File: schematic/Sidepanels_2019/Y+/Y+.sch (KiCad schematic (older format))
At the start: 42 parts, among them J1 Conn_01x04, J2 Conn_01x02

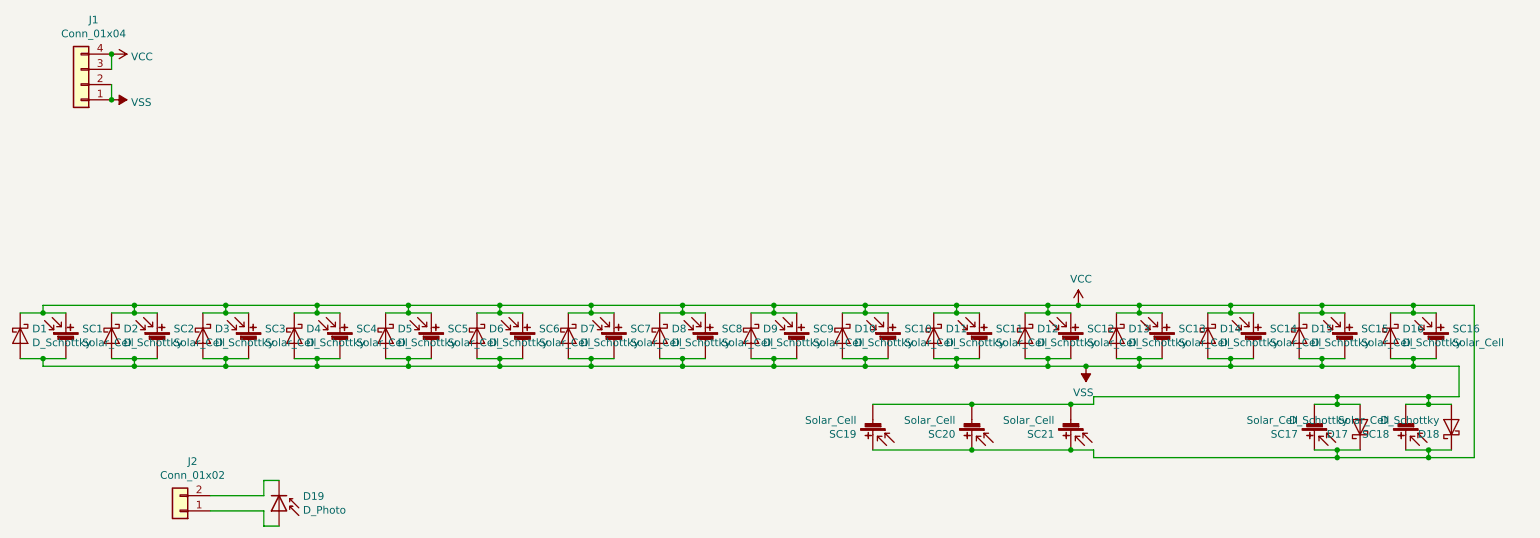
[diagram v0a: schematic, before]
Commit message: Update to Y+
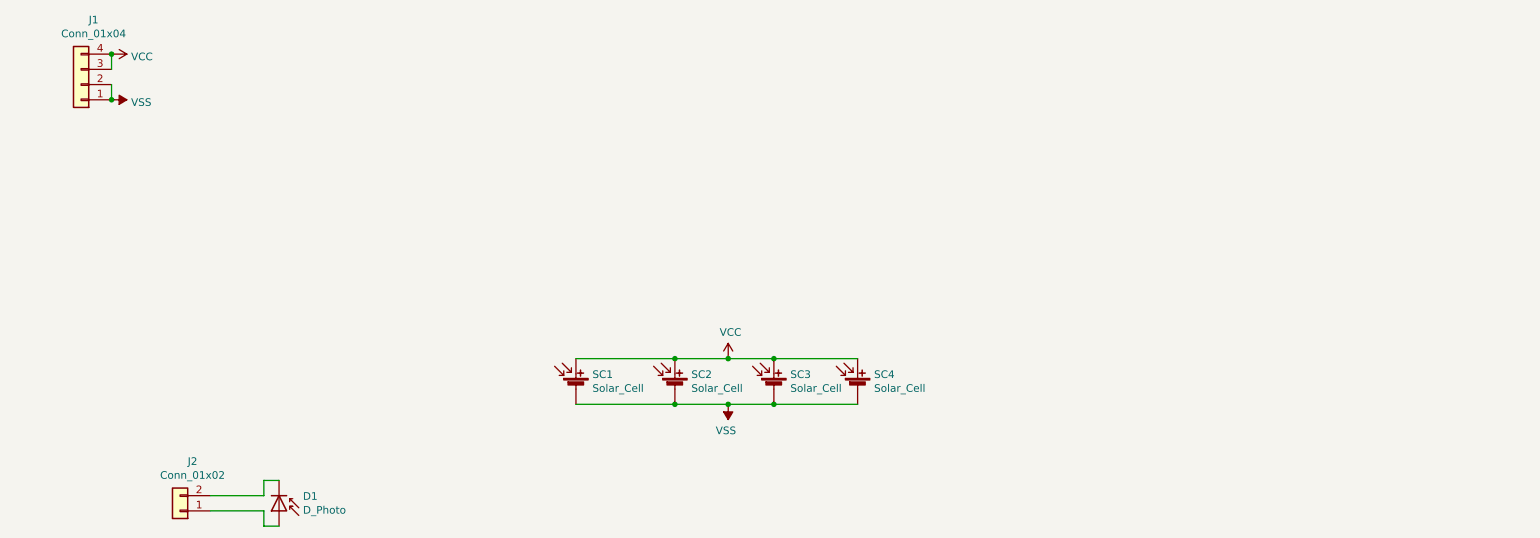
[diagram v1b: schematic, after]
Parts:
- removed D1, D10, D11, D12, D13, D14, D15, D16, D17, D18, D2, D3, D4, D5, D6, D7, D8, D9: D_Schottky, CySat footprints:Toshiba_CUS08F30, symbol Device:D_Schottky
- removed SC1, SC10, SC11, SC12, SC13, SC14, SC15, SC16, SC17, SC18, SC2, SC3, SC5, SC6, SC7, SC8, SC9: Solar_Cell, CySat footprints:TriSelectSolarPanel, symbol Device:Solar_Cell
- D1: renamed from D19; footprint CySat footprints:Sun_Sensor -> Diode_SMD:D_0805_2012Metric
- SC1: renamed from SC19; footprint CySat footprints:Spectrolab -> CySat_Solar:Spectrolab
- SC2: renamed from SC20; footprint CySat footprints:Spectrolab -> CySat_Solar:Spectrolab
- SC3: renamed from SC21; footprint CySat footprints:Spectrolab -> CySat_Solar:Spectrolab
- SC4: footprint CySat footprints:TriSelectSolarPanel -> CySat_Solar:Spectrolab
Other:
- moved on the sheet: SC1, SC2, SC3
